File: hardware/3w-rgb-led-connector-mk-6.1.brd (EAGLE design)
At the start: 52 x 39 mm, 8 parts, among them U1 SHEELD, U2 ADAFRUIT_9DOF_BREAKOUTHOLEY, U3 ADAFRUIT_BLE_UARTHOLEY-MOLEY

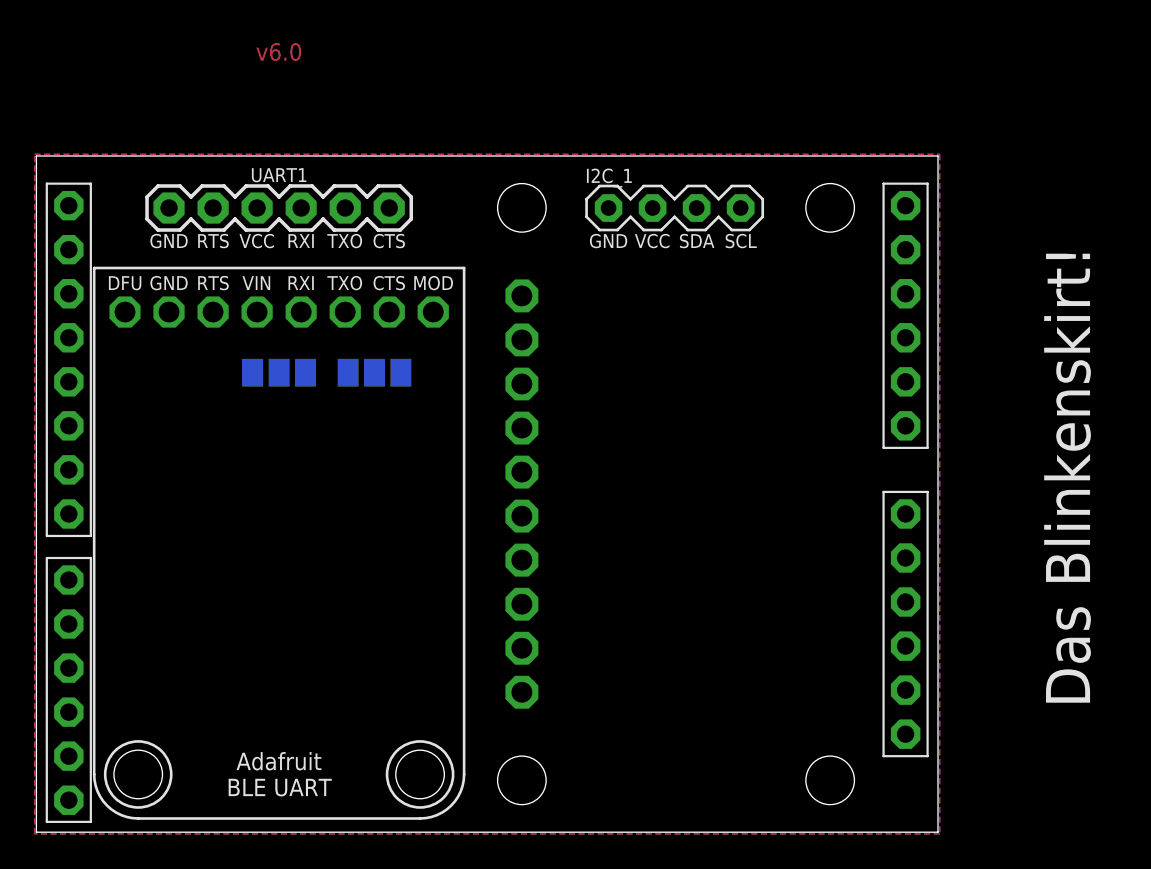
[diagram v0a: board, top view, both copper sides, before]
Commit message: dotstarstick
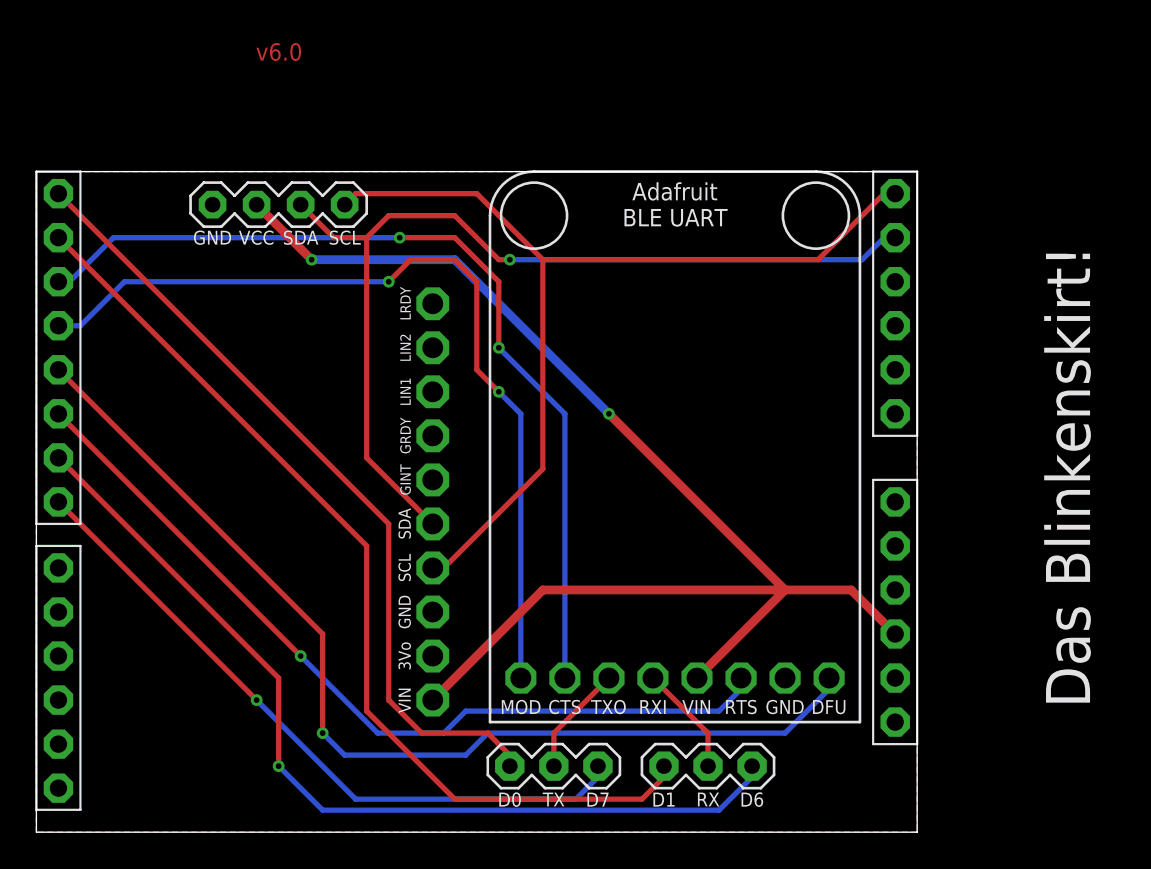
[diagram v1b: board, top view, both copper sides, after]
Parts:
- removed RXI, TXO: (no value), A_butts:PAD-JUMPER-3-NO_YES_SILK_FULL_BOX
- removed UART1: M06-UARTPTH-0.1IN, A_butts:1X06_PTH_UART
- added RX, TX: M03PTH-CENTERED, A_butts:1X03-CENTERED
- FRAME1: value (none) -> FRAME-LETTERNO_PACKAGE
- U2: value ADAFRUIT_9DOF_BREAKOUTHOLEY -> ADAFRUIT_9DOF_BREAKOUT; device A_butts:ADAFRUIT_9DOF_BREAKOUT_HOLEY -> A_butts:ADAFRUIT_9DOF_BREAKOUT
- U3: value ADAFRUIT_BLE_UARTHOLEY-MOLEY -> BLE_UART; device A_butts:ADAFRUIT_BLE_UART_HOLEY -> A_butts:ADAFRUIT_BLE_UART_NOTHOLEY
- moved U3 31.1 mm to (36.8, 8.89), turned to 0 degrees
- moved I2C_1 22.8 mm to (10.2, 36.2)
- moved U2 5.16 mm to (22.9, 19.1), flipped to the top
- moved U1 0.92 mm to (1.27, 36.8)
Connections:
- removed net D2: U1.D2, U3.CTS, UART1.CTS
- removed net D5: U1.D5, U3.RTS, UART1.RTS
- removed net D8: U1.D8, U3.MOD
- new net CTS: U1.D2, U3.CTS
- new net MOD: U1.D3, U3.MOD
- new net RTS: U1.D5, U3.RTS
- net 5V: no longer UART1.VCC
- net D6: now also RX.1; no longer RXI.3
- net D7: now also TX.1; no longer TXO.3
- net GND: no longer UART1.GND
- net RX: now also TX.3; no longer TXO.1
- net RXI: now also RX.2; no longer RXI.2, UART1.RXI
- net SCL: now also I2C_1.SCL; no longer I2C_1.SDA
- net SDA: now also I2C_1.SDA; no longer I2C_1.SCL
- net TX: now also RX.3; no longer RXI.1
- net TXO: now also TX.2; no longer TXO.2, UART1.TXO
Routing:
- net 5V: track 0.00 -> 77.2 mm, vias 0 -> 2
- net D4: track 0.00 -> 59.2 mm, vias 0 -> 1
- net SCL: track 0.00 -> 56.0 mm
- net SDA: track 0.00 -> 55.3 mm, vias 0 -> 1
- net TX: track 0.00 -> 55.1 mm
- net D6: track 0.00 -> 52.8 mm, vias 0 -> 1
- net CTS: track 0.00 -> 51.9 mm, vias 0 -> 2
- net MOD: track 0.00 -> 50.1 mm, vias 0 -> 2
- net RTS: track 0.00 -> 48.7 mm, vias 0 -> 1
- net RX: track 0.00 -> 46.0 mm
- net D7: track 0.00 -> 39.4 mm, vias 0 -> 1
- net TXO: track 0.00 -> 6.40 mm
- net RXI: track 0.00 -> 6.40 mm
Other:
- board size 52 x 39 mm -> 50.8 x 38.1 mm
